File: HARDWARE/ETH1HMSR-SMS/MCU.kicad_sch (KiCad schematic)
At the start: 33 parts, among them J401 20021111-00010T4LF, U401 STM32H743VITx, U402 24LC08B-E/MS, U403 ADR4533, Y401 NX5032GA-16

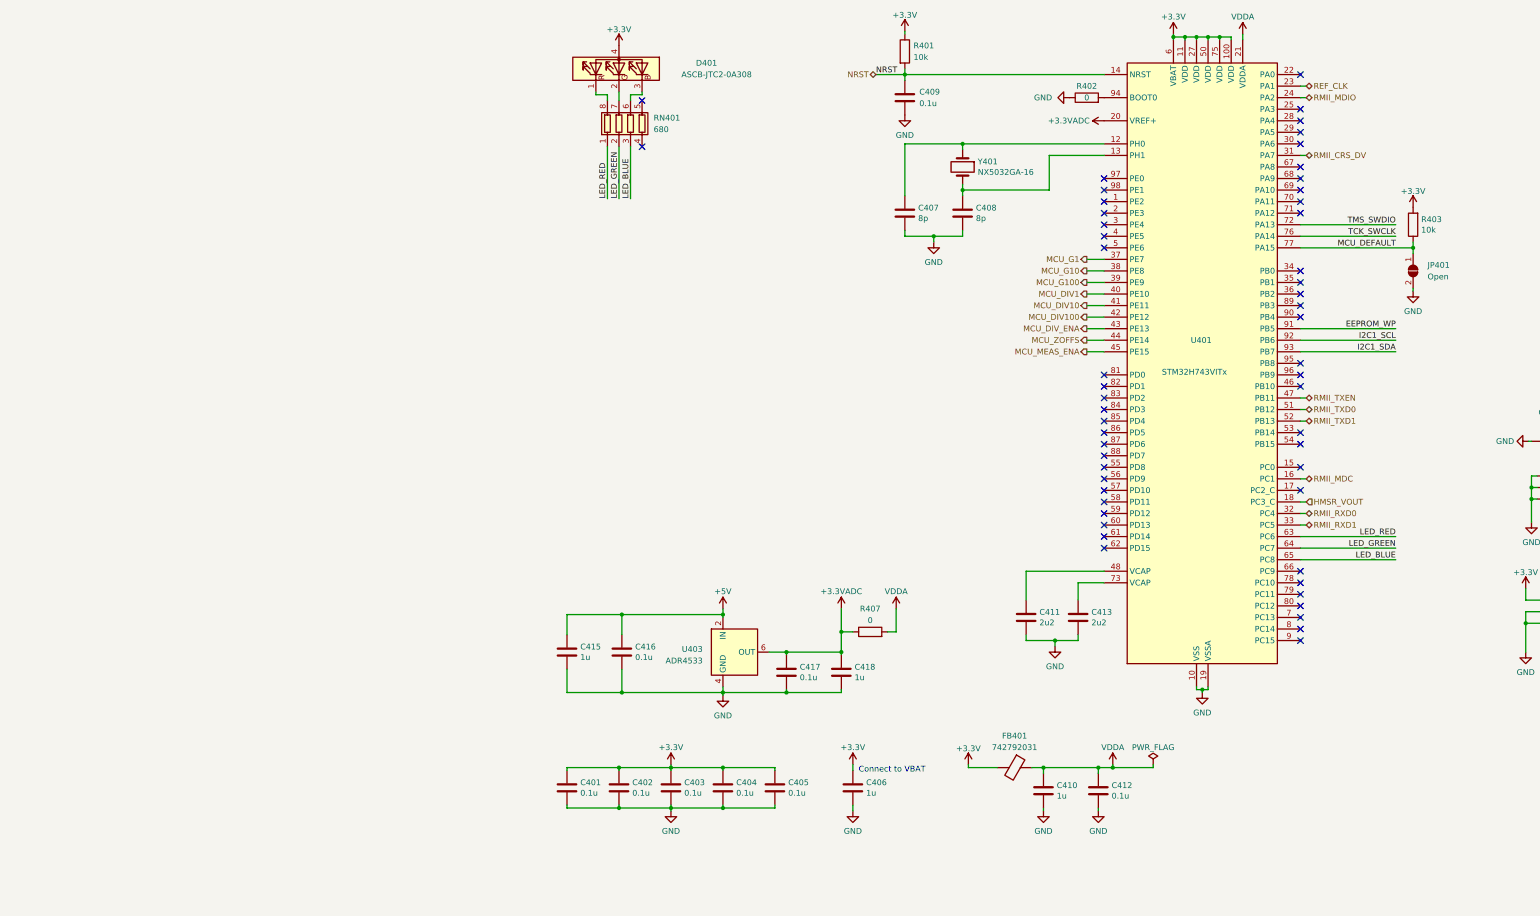
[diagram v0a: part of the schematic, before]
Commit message: PCB design
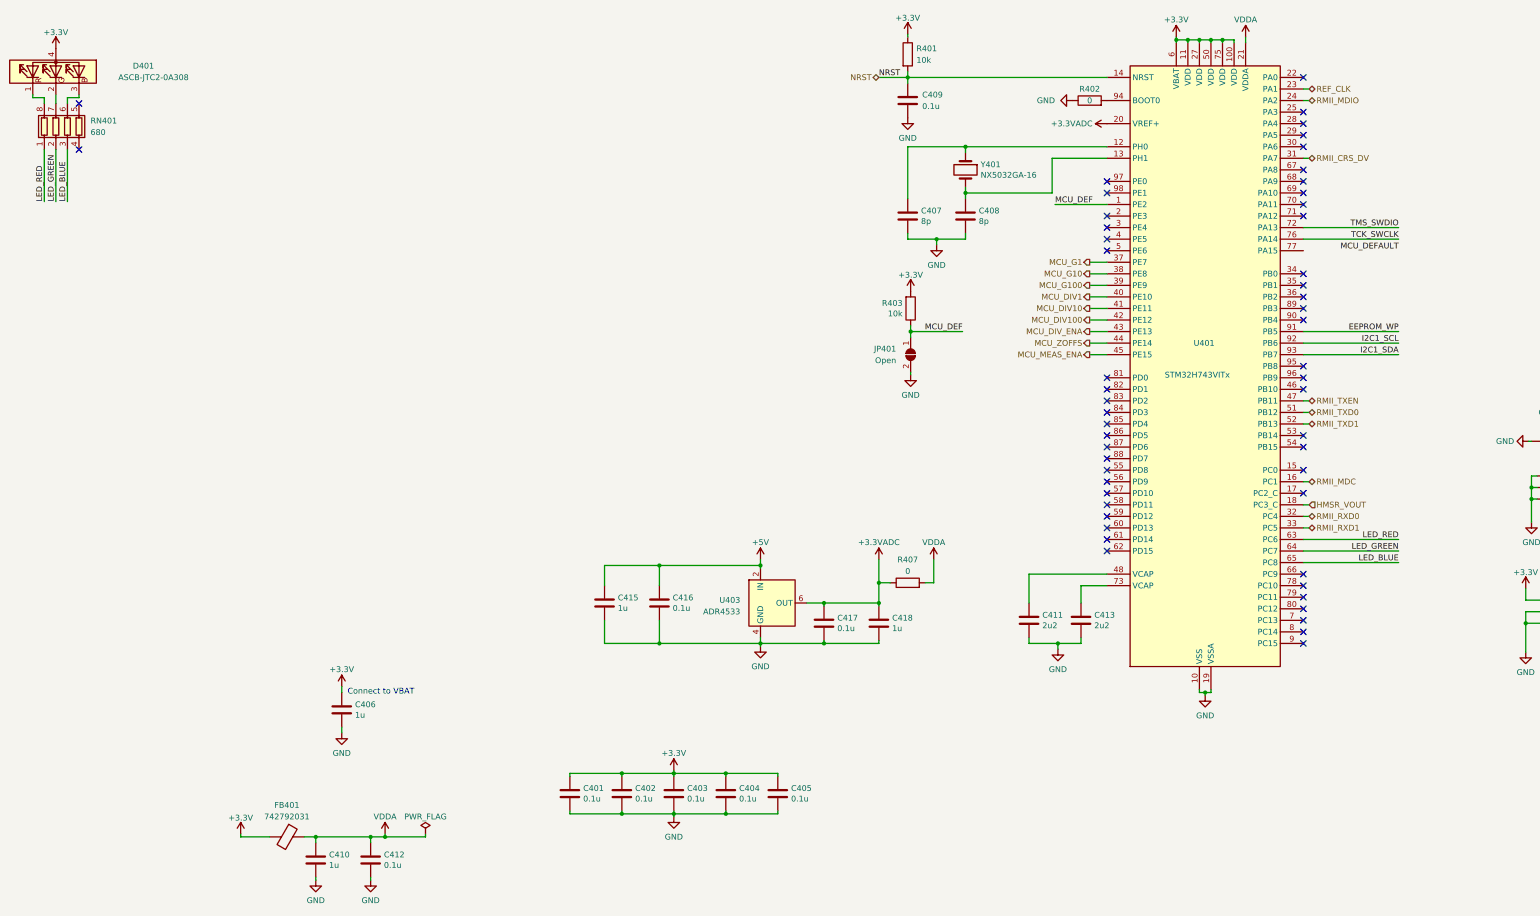
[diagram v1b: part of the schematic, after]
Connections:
- net MCU_DEFAULT: no longer JP401.1 (A), R403.1, U401.77 (PA15)
- net MCU_DEF: now reaches U401.1 (PE2)
- net MCU_DEF: now also JP401.1 (A), R403.1
- no-connect marks 58 -> 57
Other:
- moved on the sheet: C401, C402, C403, C404, C405, C406, C407, C408, C409, C410, C411, C412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
